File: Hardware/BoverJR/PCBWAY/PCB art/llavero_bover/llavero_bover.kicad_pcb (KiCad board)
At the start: 2 copper layers, 28.8 x 35.9 mm, 2 parts

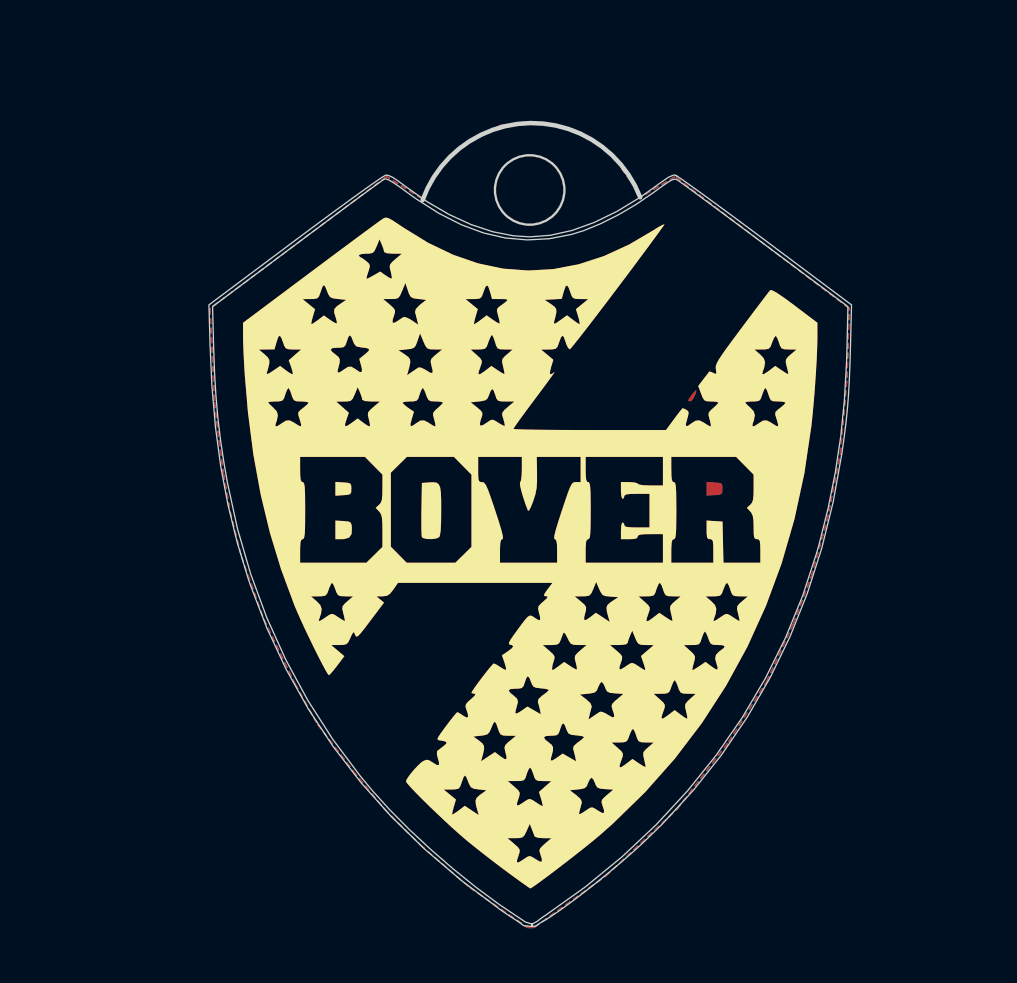
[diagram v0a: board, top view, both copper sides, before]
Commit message: CASI TERMINO LLAVERO BOVER
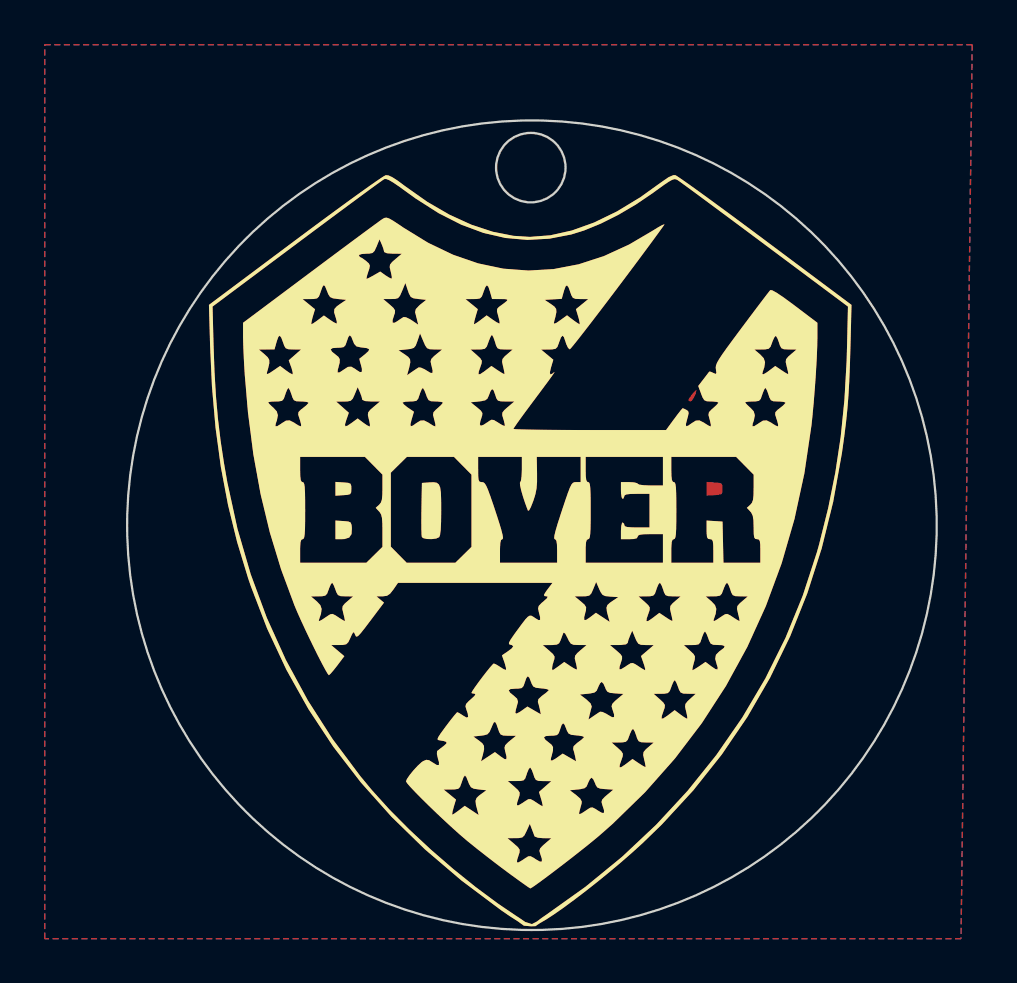
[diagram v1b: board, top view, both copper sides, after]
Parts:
- moved H1 1.00 mm to (127.2, 84.5)
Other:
- board size 28.8 x 35.9 mm -> 36.2 x 36.2 mm
